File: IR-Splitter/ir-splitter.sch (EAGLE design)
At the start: 40 parts, among them Q1 BC447, Q2 BC557B, T1 IRFR024N, T10 IRFR024N, T2 IRFR024N, T3 IRFR024N, T4 IRFR024N, T5 IRFR024N, T6 IRFR024N, T7 IRFR024N, T8 IRFR024N, T9 IRFR024N

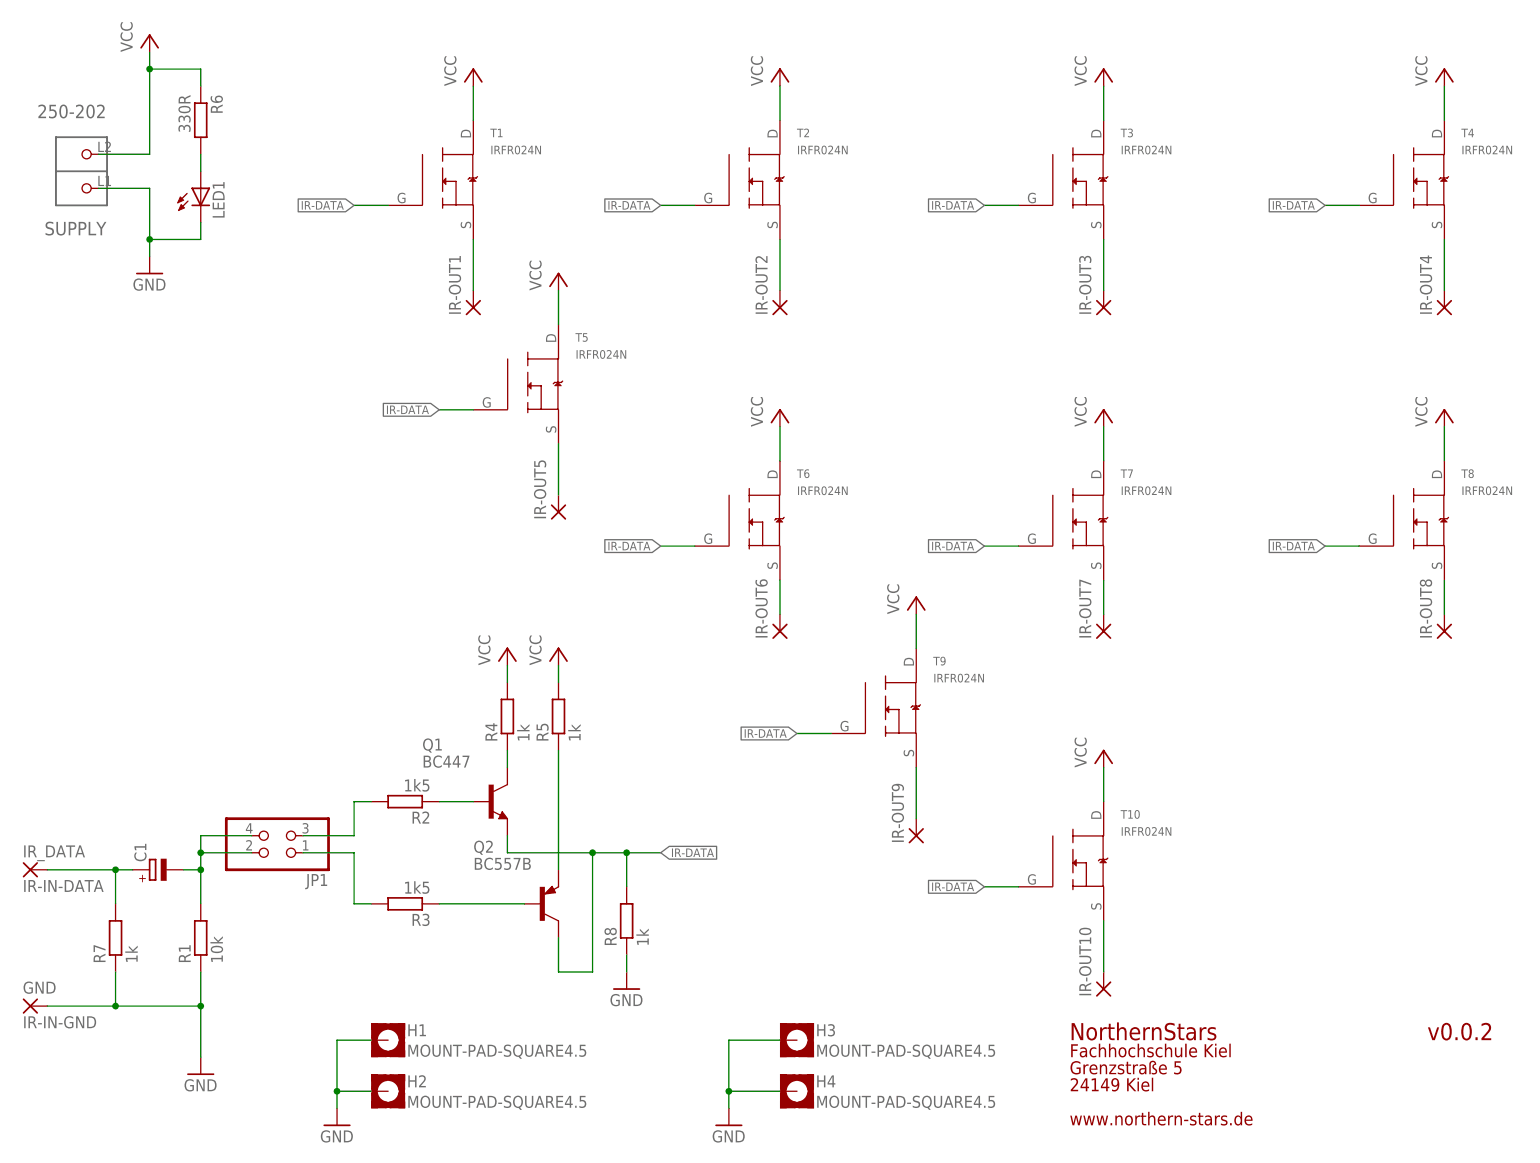
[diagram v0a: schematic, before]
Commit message: Updated IR-Splitter to Version 1.0.0
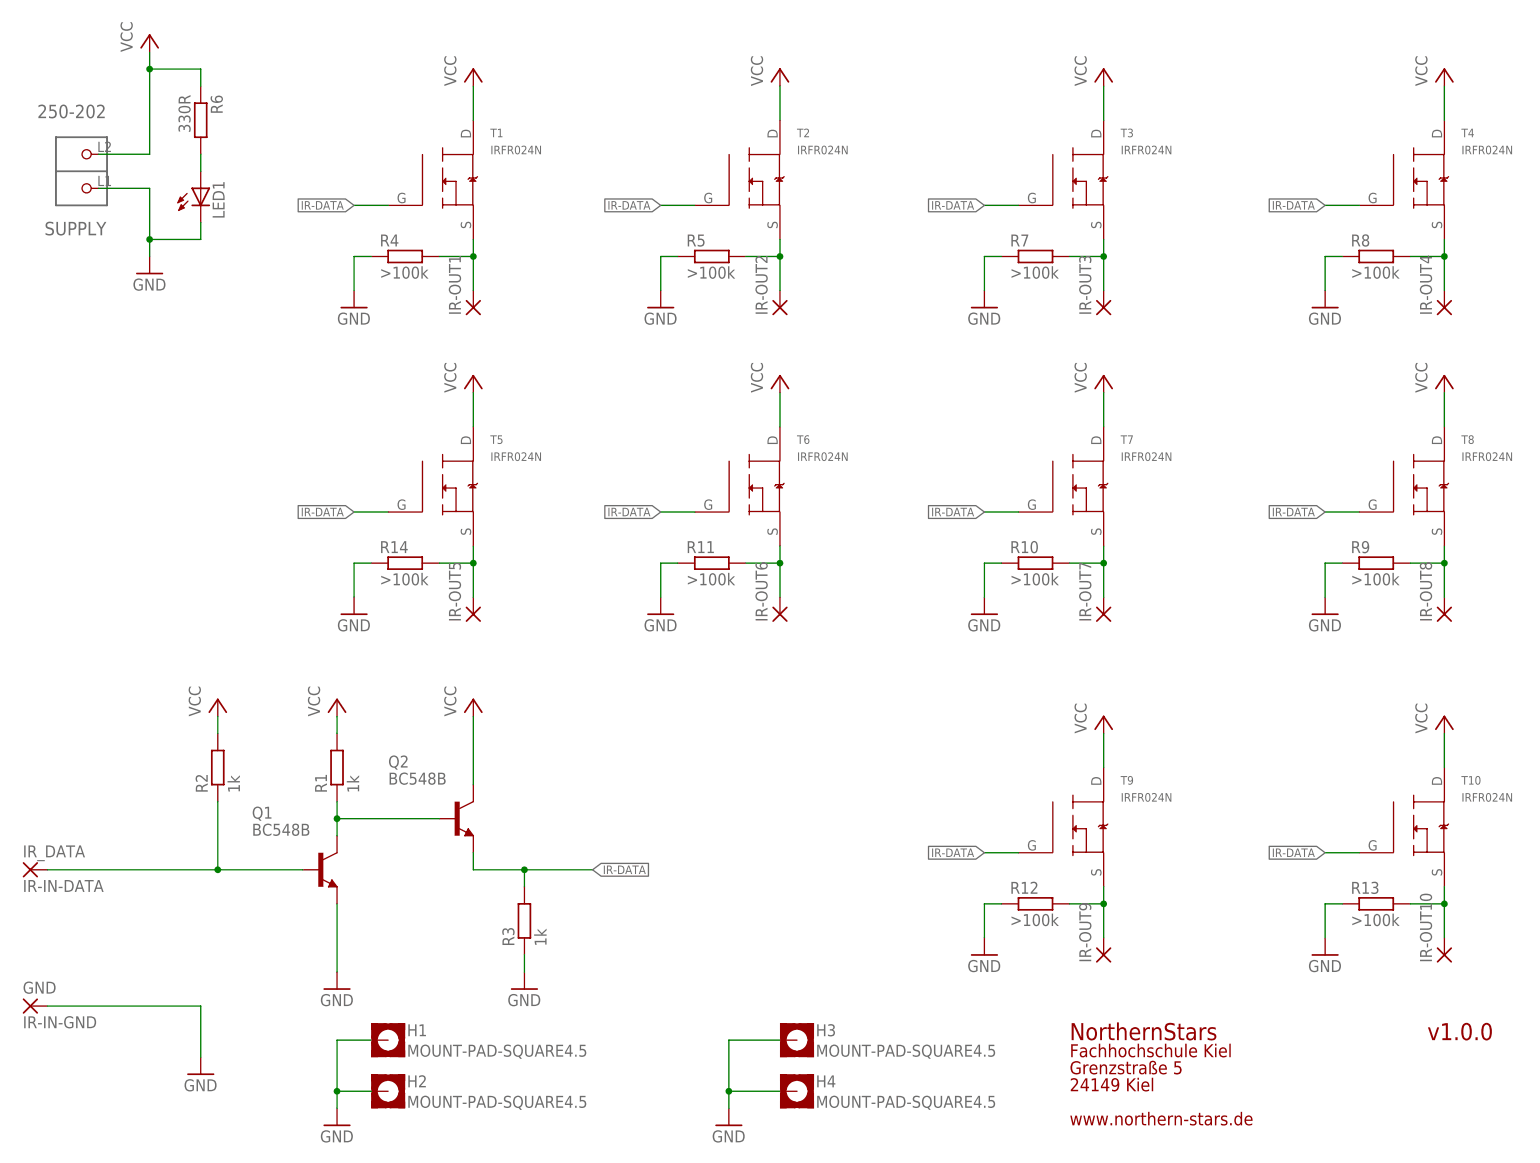
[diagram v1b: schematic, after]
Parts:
- removed C1: (no value), rcl:CPOL-EUE2.5-5
- removed JP1: (no value), pinhead-2:PINHD-2X02_2.54-SMD
- added R10, R11, R12, R13, R14, R9: >100k, rcl:R-EU_R1206
- LED1: device led:LED3MM -> led:LEDCHIPLED_1206
- Q1: value BC447 -> BC548B; device transistor-npn:BC447 -> transistor-npn:BC548B
- Q2: value BC557B -> BC548B; device transistor-pnp:BC557B -> transistor-npn:BC548B
- R1: value 10k -> 1k; device rcl:R-EU_0207/10 -> rcl:R-EU_R1206
- R2, R3: value 1k5 -> 1k; device rcl:R-EU_0207/10 -> rcl:R-EU_R1206
- R4, R5, R7, R8: value 1k -> >100k; device rcl:R-EU_0207/10 -> rcl:R-EU_R1206
- R6: device rcl:R-EU_0207/10 -> rcl:R-EU_R1206
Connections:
- removed net DATA: C1.-, JP1.2, JP1.4, R1.2
- removed net N$12: Q1.C, R4.1
- removed net N$13: Q2.E, R5.1
- removed net N$14: Q2.B, R3.1
- removed net N$17: JP1.3, R2.2
- removed net N$18: JP1.1, R3.2
- net GND: now also Q1.E, R10.1, R11.1, R12.1, R13.1, R14.1, R3.1, R4.1, R5.1, R9.1; no longer R1.1
- net IR-DATA: now also Q2.E, R3.2; no longer Q1.E, Q2.C, R8.2
- net N$1: now also R4.2
- net N$10: now also R12.2
- net N$11: now also Q1.C, Q2.B, R1.1; no longer Q1.B, R2.1
- net N$16: now also Q1.B, R2.1; no longer C1.+, R7.2
- net N$2: now also R5.2
- net N$3: now also R14.2
- net N$4: now also R11.2
- net N$5: now also R9.2
- net N$6: now also R10.2
- net N$7: now also R8.2
- net N$8: now also R7.2
- net N$9: now also R13.2
- net VCC: now also Q2.C, R1.2, R2.2; no longer R4.2, R5.2
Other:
- note added: "v1.0.0"
- note removed: "v0.0.2"
- moved on the sheet: IR-OUT10, IR-OUT5, IR-OUT6, IR-OUT7, IR-OUT8, IR-OUT9, Q1, R1, R2, R3, R4, R5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
